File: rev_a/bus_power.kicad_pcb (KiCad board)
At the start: 2 copper layers, 50 x 50 mm, 14 parts, among them Q1 FQP47P06, Q2 FQP47P06, SW1 F-426-0020

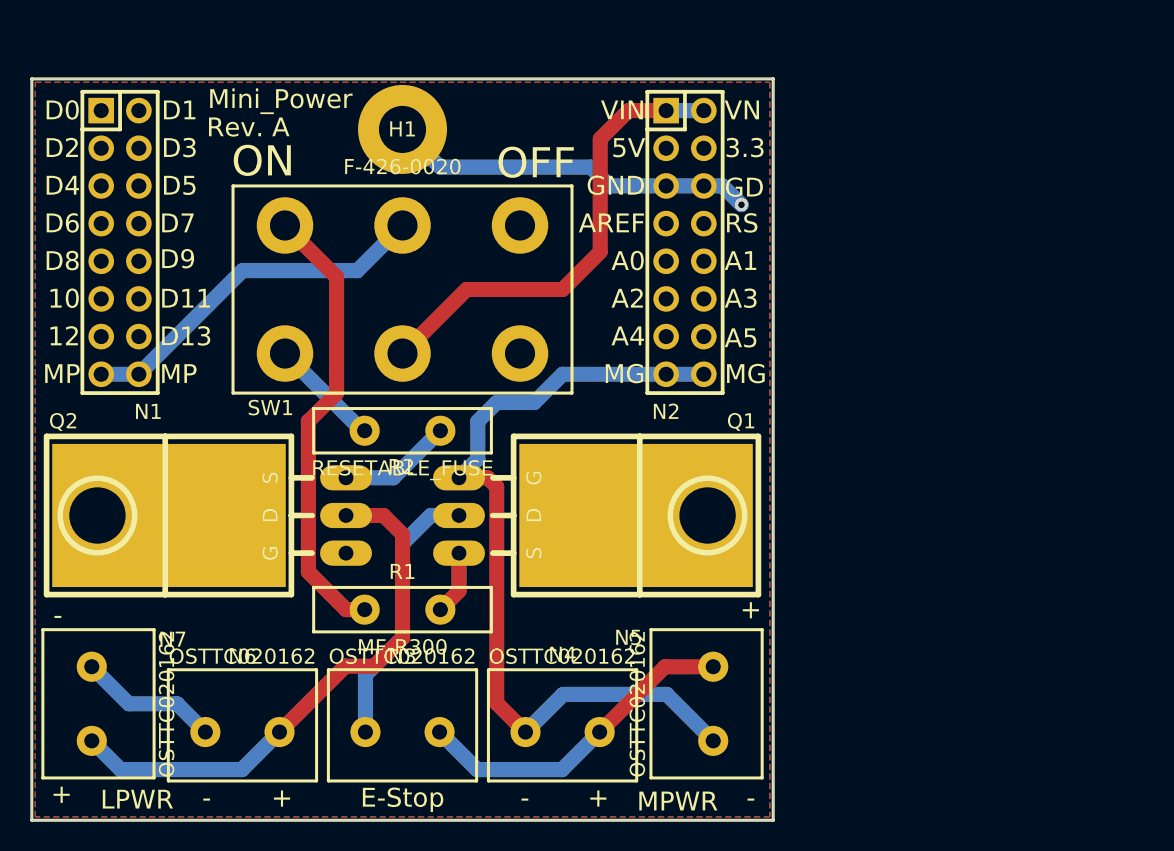
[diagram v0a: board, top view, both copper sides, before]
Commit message: Finnished Revision A layout.
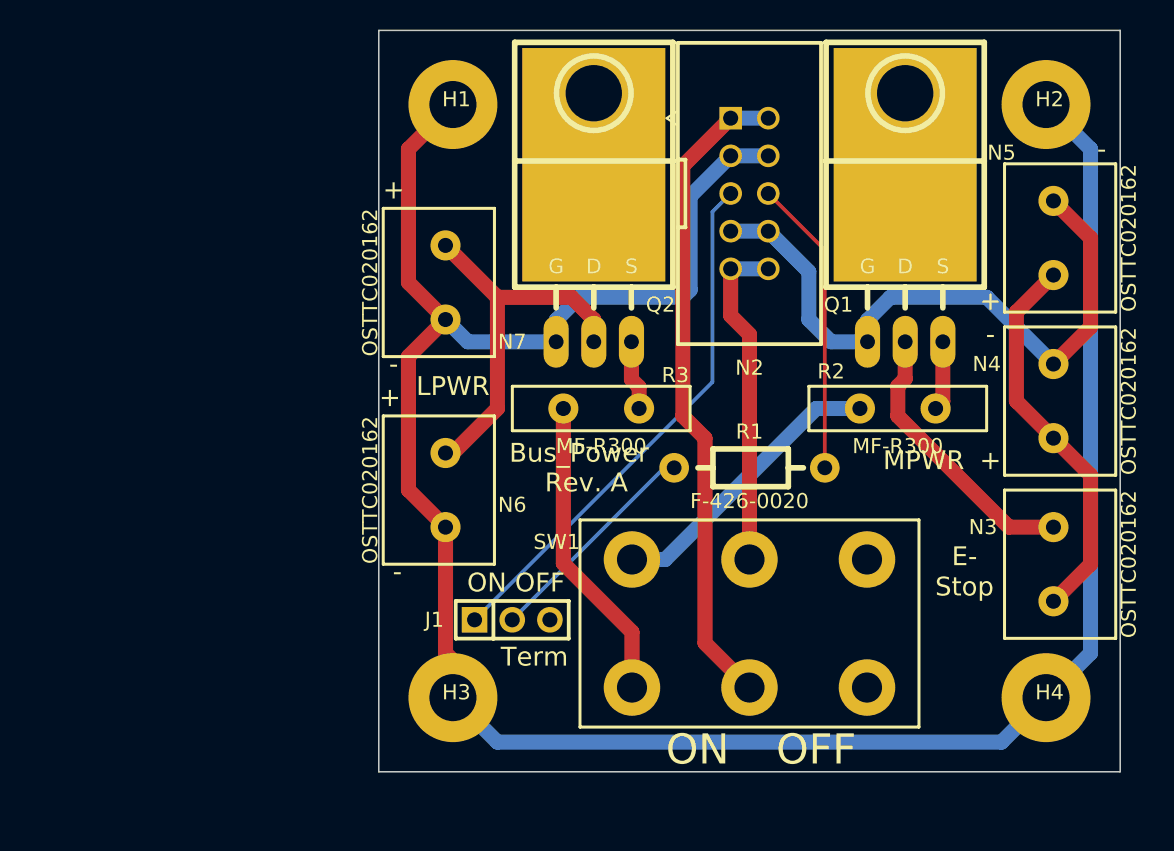
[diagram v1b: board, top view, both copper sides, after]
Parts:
- removed N1: MS_DATA_HEADER_POWER, Mini_Power_Rev_A:Pin_Header_Straight_2x08
- added H2: 3MM_HOLE, Bus_BeagleBone_Rev_A:MountingHole_3mm, F.Cu at (145.0, 105.0)
- added H3: 3MM_HOLE, Bus_BeagleBone_Rev_A:MountingHole_3mm, F.Cu at (105.0, 145.0)
- added H4: 3MM_HOLE, Bus_BeagleBone_Rev_A:MountingHole_3mm, F.Cu at (145.0, 145.0)
- added J1: TERMINATE_JUMPER, Bus_BeagleBone_Rev_A:Pin_Header_Straight_1x03, F.Cu at (109.0, 139.8)
- added R3: MF-R300, Bus_Power_Rev_A:MF_R300, F.Cu at (115.0, 125.5)
- G1: footprint Mini_Power_Rev_A:OSHW_LOGO_400mil -> Bus_BeagleBone_Rev_A:OSHW_LOGO_400mil
- H1: footprint Mini_Power_Rev_A:MountingHole_3mm -> Bus_BeagleBone_Rev_A:MountingHole_3mm
- N2: value MS_PWR_HEADER_POWER -> BUS_MASTER_HEADER; footprint Mini_Power_Rev_A:Pin_Header_Straight_2x08 -> Bus_BeagleBone_Rev_A:Pin_Header_Straight_2x05_Shrouded
- N3, N4, N5, N6, N7: footprint Mini_Power_Rev_A:5MM_TERMINAL_BLOCK_2_POS -> Bus_BeagleBone_Rev_A:5MM_TERMINAL_BLOCK_2_POS
- Q1, Q2: footprint Mini_Power_Rev_A:TO-220_FET-GDS_Horizontal_LargePads -> Bus_BeagleBone_Rev_A:TO-220_FET-GDS_Horizontal_LargePads
- R1: value MF-R300 -> 120 1%; footprint Mini_Power_Rev_A:MF_R300 -> Bus_BeagleBone_Rev_A:Resistor_Horizontal__400
- R2: value RESETABLE_FUSE -> MF-R300; footprint Mini_Power_Rev_A:MF_R300 -> Bus_Power_Rev_A:MF_R300
- SW1: footprint Mini_Power_Rev_A:GF_426_0020 -> Bus_Power_Rev_A:GF_426_0020
- moved G1 54.0 mm to (138.8, 110.5)
- moved N3 45.3 mm to (145.5, 136.0), turned to 270 degrees
- moved N4 39.9 mm to (145.5, 125.0), turned to 270 degrees
- moved N5 38.9 mm to (145.5, 114.0), turned to 270 degrees
- moved N7 37.1 mm to (104.5, 117.0), turned to 90 degrees
- moved R2 33.4 mm to (135.0, 125.5)
- moved SW1 32.5 mm to (125.0, 140.0)
- moved Q1 32.3 mm to (135.5, 121.0), turned to 0 degrees
- moved R1 25.3 mm to (125.0, 129.5), turned to 0 degrees
- moved N6 21.3 mm to (104.5, 131.0), turned to 90 degrees
- moved Q2 20.4 mm to (114.5, 121.0), turned to 0 degrees
- moved N2 5.46 mm to (125.0, 111.0)
- moved H1 3.79 mm to (105.0, 105.0)
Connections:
- net /MPWR1 renamed /BPWR2
- H1 pad 1: /GND -> /LGND
- N2 pad 1: /VIN -> /LPWR4
- N2 pad 10: (no net) -> /BPWR5
- N2 pad 2: /VIN -> /LPWR4
- N2 pad 3: (no net) -> /LGND
- N2 pad 4: (no net) -> /LGND
- N2 pad 5: /GND -> /CANH
- N2 pad 6: /GND -> /CANL
- N2 pad 7: (no net) -> /BGND
- N2 pad 8: (no net) -> /BGND
- N2 pad 9: (no net) -> /BPWR5
- N3 pad 2: /LPWR4 -> /BPWR1
- N4 pad 1: /MGND -> /BGND
- N4 pad 2: /LPWR4 -> /BPWR1
- N5 pad 1: /MGND -> /BGND
- N5 pad 2: /LPWR4 -> /BPWR1
- N6 pad 1: /GND -> /LGND
- N7 pad 1: /GND -> /LGND
- Q1 pad G: /MGND -> /BGND
- Q1 pad S: /MPWR2 -> /BPWR3
- Q2 pad G: /GND -> /LGND
- R1 pad 1: /MPWR2 -> Net-(J1-Pad2)
- R1 pad 2: /MPWR3 -> /CANL
- R2 pad 1: /LPWR2 -> /BPWR3
- R2 pad 2: /LPWR3 -> /BPWR4
- SW1 pad 1: /MPWR3 -> /BPWR4
- SW1 pad 2: /MPWR -> /BPWR5
- SW1 pad 3: (no net) -> Net-(SW1-Pad3)
- SW1 pad 5: /VIN -> /LPWR4
- SW1 pad 6: (no net) -> Net-(SW1-Pad6)
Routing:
- net /LGND: track 0.00 -> 161.7 mm
- net /MGND: track 57.0 -> 0.00 mm
- net /BGND: track 0.00 -> 43.8 mm
- net /CANH: track 0.00 -> 35.9 mm
- net /GND: track 34.4 -> 0.00 mm, vias 1 -> 0
- net /VIN: track 31.6 -> 0.00 mm
- net /MPWR3: track 30.4 -> 0.00 mm
- net /BPWR1: track 0.00 -> 26.1 mm
- net /MPWR: track 24.5 -> 0.00 mm
- net /BPWR5: track 0.00 -> 22.7 mm
- net /LPWR4: track 22.4 -> 44.1 mm
- net /CANL: track 0.00 -> 20.1 mm
- net /BPWR4: track 0.00 -> 19.6 mm
- net Net-(J1-Pad2): track 0.00 -> 15.2 mm
- net /LPWR3: track 7.53 -> 20.7 mm
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- removed copper zone on B.Cu, net /GND
- removed copper zone on F.Cu, net /GND
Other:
- board text added: "Bus Power Rev. A 11Aug2014 (c) Gramlich"
- board text added: "Bus_Power"
- board text added: "E- Stop"
- board text added: "ON OFF"
- board text added: "Term"
- board text removed: "10"
- board text removed: "12"
- board text removed: "3.3"
- board text removed: "5V"
- board text removed: "A0"
- board text removed: "A1"
- board text removed: "A2"
- board text removed: "A3"
- board text removed: "A4"
- board text removed: "A5"
- board text removed: "AREF"
- board text removed: "D0"
- board text removed: "D1"
- board text removed: "D11"
- board text removed: "D13"
- board text removed: "D2"
- board text removed: "D3"
- board text removed: "D4"
- board text removed: "D5"
- board text removed: "D6"
- board text removed: "D7"
- board text removed: "D8"
- board text removed: "D9"
- board text removed: "E-Stop"
- board text removed: "GD"
- board text removed: "GND"
- board text removed: "MG"
- board text removed: "MP"
- board text removed: "Mini_Power"
- board text removed: "Power Mini-Shield Rev. A Copyright (c) 2014 - Gramlich"
- board text removed: "RS"
- board text removed: "VIN"
- board text removed: "VN"
